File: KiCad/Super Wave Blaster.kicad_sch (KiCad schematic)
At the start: 21 parts, among them J1 EIAJ_Input, J2 PCM5102_I2S, J3 PCM5102_Audio, J4 Power Input, J5 Audio_Jack, J6 Power Input, J7 Audio Out, U1 TLV73333PDBV, U2 CD74HCT14PWR, U3 SN74HC595PWR, U4 SN74LVC8T245PWR

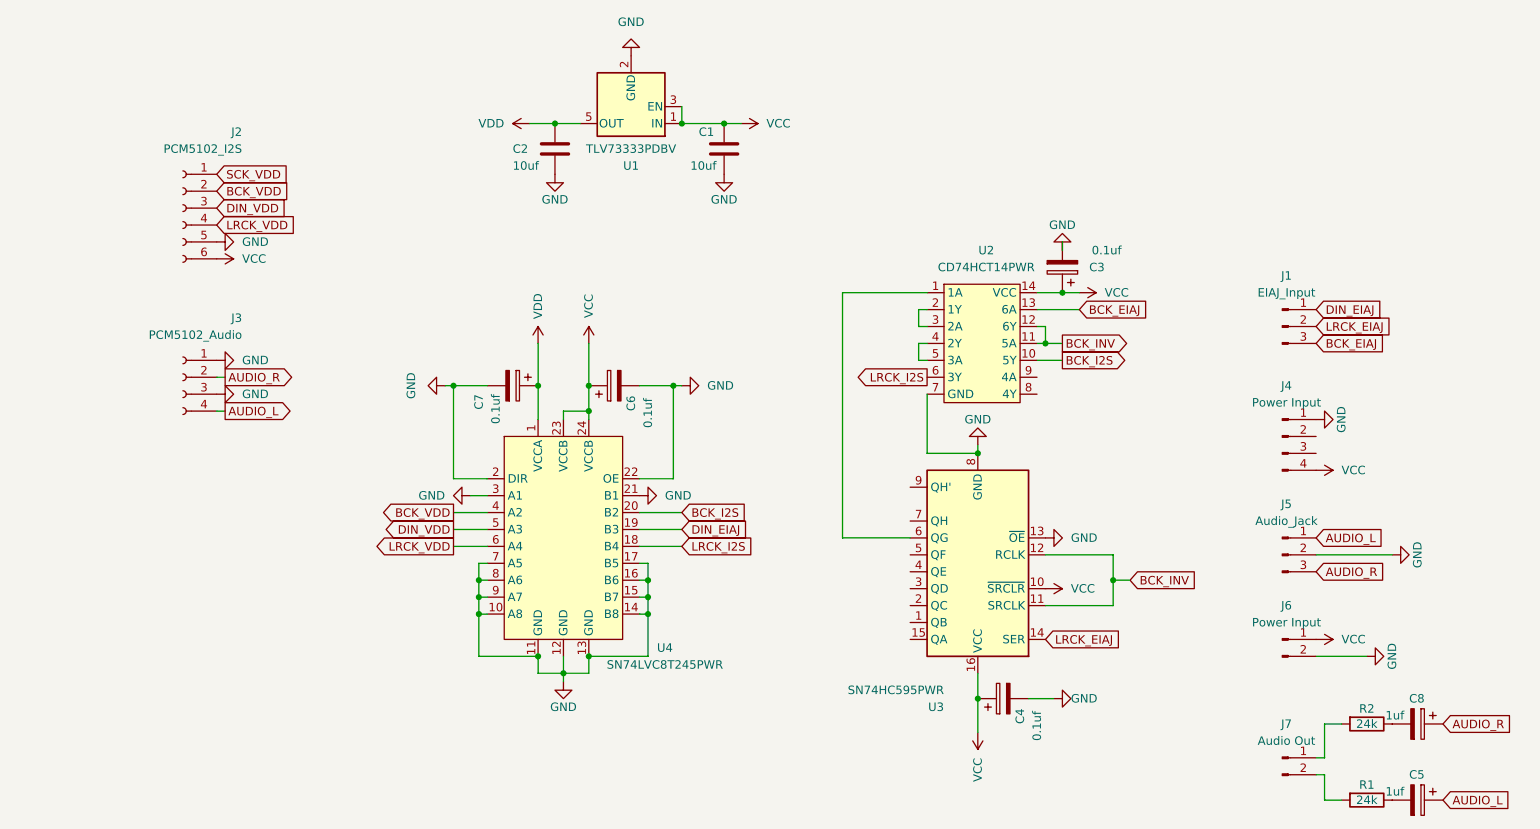
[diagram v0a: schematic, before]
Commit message: Cleanup schematic layout
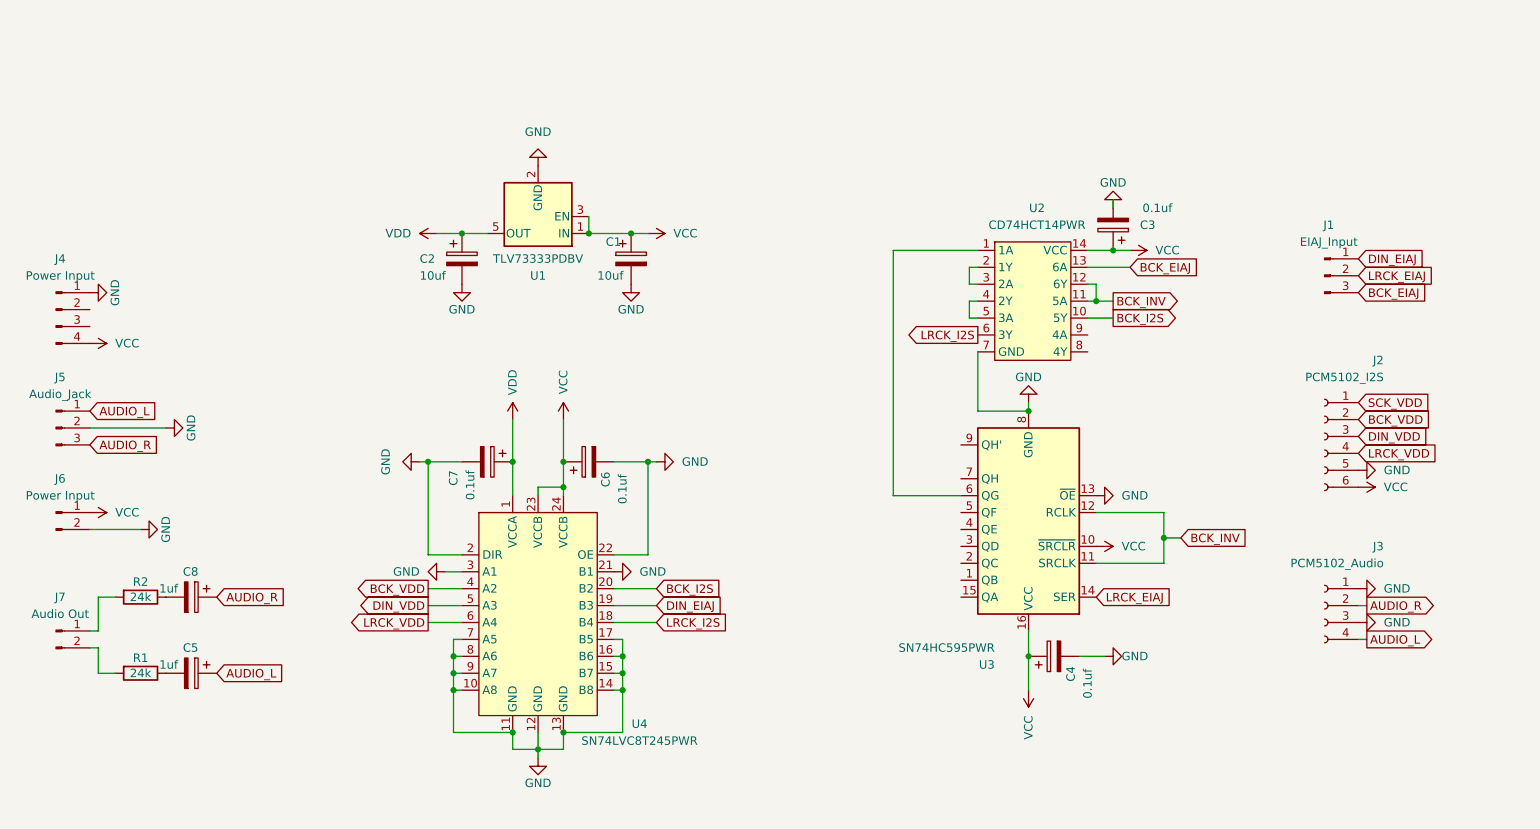
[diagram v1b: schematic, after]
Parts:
- C1, C2: symbol Device:C -> Device:C_Polarized
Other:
- moved on the sheet: C3, C4, C5, C6, C7, C8, J1, J2, J3, J4, J5, J6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
